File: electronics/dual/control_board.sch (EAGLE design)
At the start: 136 parts, among them J17 JST_PH_B3B-PH-K-S(LF)(SN), J18 JST_PH_B3B-PH-K-S(LF)(SN), J19 JST_PH_B3B-PH-K-S(LF)(SN), J20 JST_PH_B3B-PH-K-S(LF)(SN), J21 JST_PH_B3B-PH-K-S(LF)(SN), J22 JST_PH_B3B-PH-K-S(LF)(SN), J23 JST_PH_B3B-PH-K-S(LF)(SN), J24 JST_PH_B3B-PH-K-S(LF)(SN), J25 JST_PH_B3B-PH-K-S(LF)(SN), J26 JST_PH_B3B-PH-K-S(LF)(SN), J27 JST_PH_B3B-PH-K-S(LF)(SN), J28 JST_PH_B3B-PH-K-S(LF)(SN), J29 JST_PH_B3B-PH-K-S(LF)(SN), J30 JST_PH_B3B-PH-K-S(LF)(SN), J31 JST_PH_B3B-PH-K-S(LF)(SN), J32 JST_PH_B3B-PH-K-S(LF)(SN), J49 B4B-PH-K-S(LF)(SN), J50 B4B-PH-K-S(LF)(SN), J51 B4B-PH-K-S(LF)(SN), J52 B4B-PH-K-S(LF)(SN), J53 B4B-PH-K-S(LF)(SN), J54 B4B-PH-K-S(LF)(SN), J55 B4B-PH-K-S(LF)(SN), J56 B4B-PH-K-S(LF)(SN), J57 B4B-PH-K-S(LF)(SN), J58 B4B-PH-K-S(LF)(SN), J59 B4B-PH-K-S(LF)(SN), J60 B4B-PH-K-S(LF)(SN), J61 B4B-PH-K-S(LF)(SN), J62 B4B-PH-K-S(LF)(SN), J63 B4B-PH-K-S(LF)(SN), J64 B4B-PH-K-S(LF)(SN), Q1 BCF29SMD, U18 AD7730BRUZ, U19 AD5360BSTZ, U2 AMP-5103309-7-34PIN_5103309-7, U20 ADR425ARZ, U21 AD7730BRUZ, U23 AD7730BRUZ, U24 AD7730BRUZ, U25 AD7730BRUZ, U26 AD7730BRUZ, U27 AD7730BRUZ, U28 AD7730BRUZ, U4 ADR421ARZ, U5 AD7616BSTZ, X1 22-23-2031, Y1 KC2520B-C1, Y3 KC2520B-C1

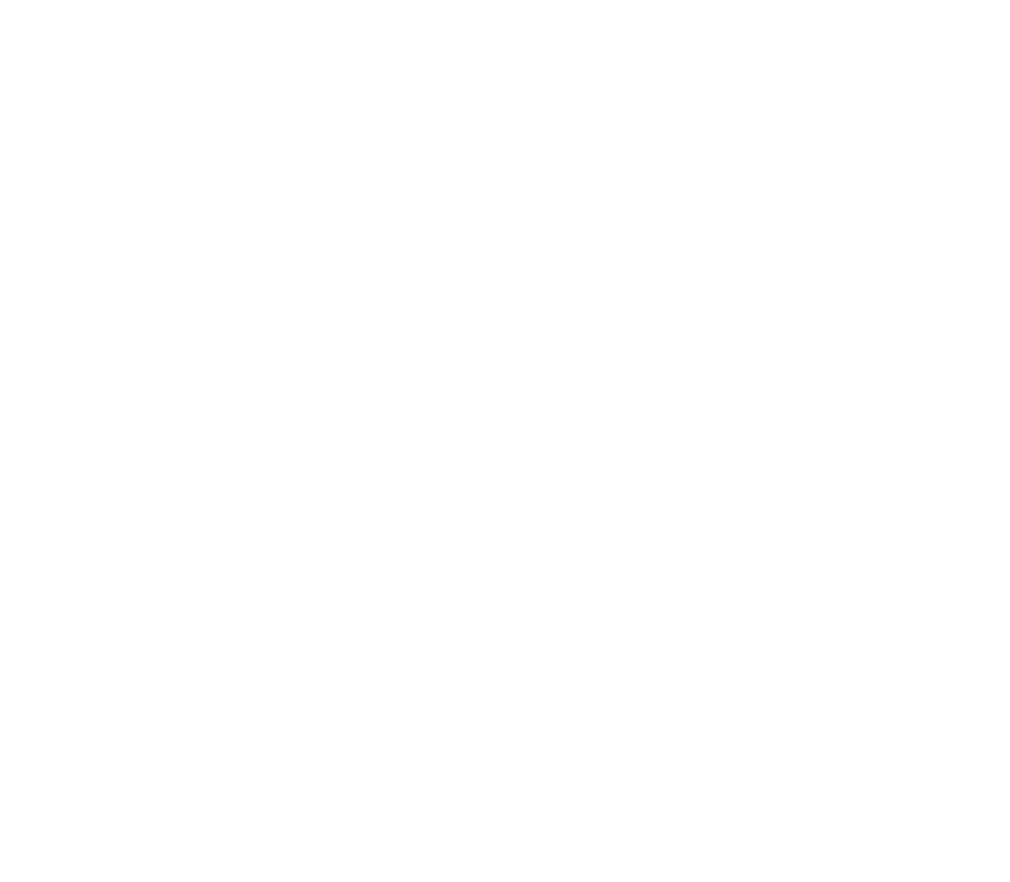
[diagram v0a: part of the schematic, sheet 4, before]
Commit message: added raspi firmware
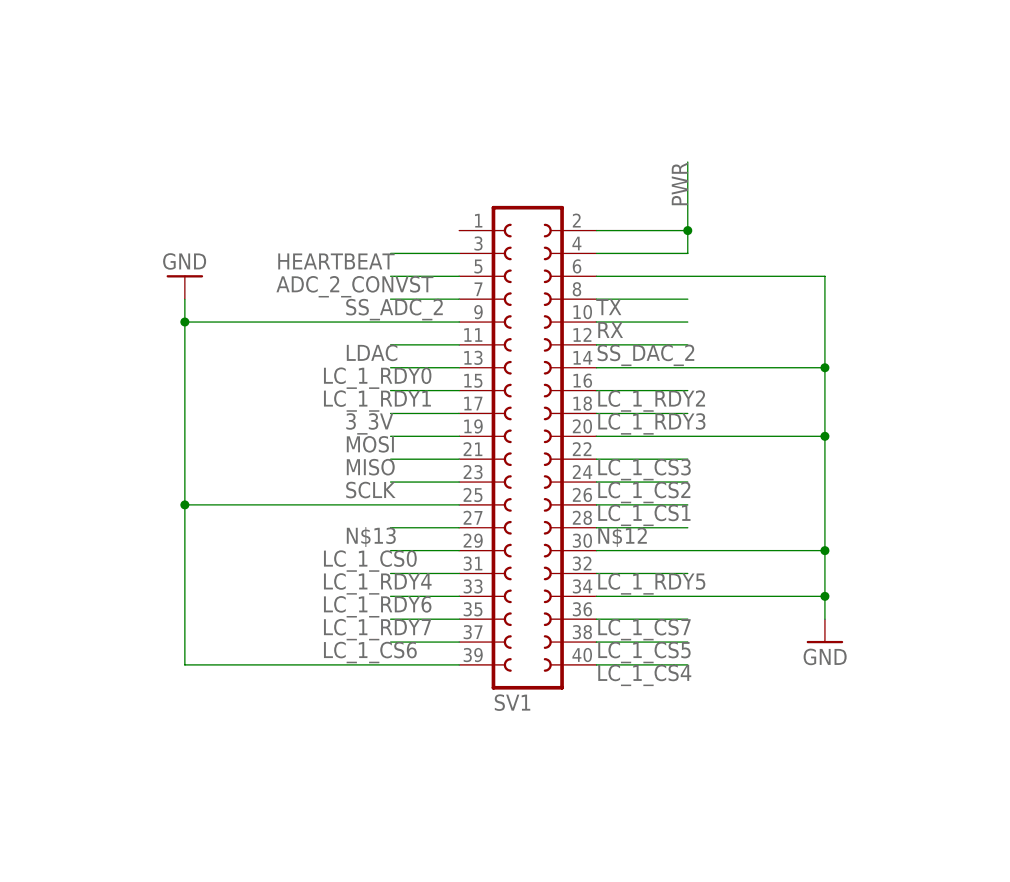
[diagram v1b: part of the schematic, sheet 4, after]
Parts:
- added SV1: (no value), con-lsta:FE20-2
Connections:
- new net 3_3V: SV1.17
- new net N$12: SV1.28
- new net N$13: SV1.27
- net ADC_2_CONVST: now also SV1.5
- net GND: now also SV1.14, SV1.20, SV1.25, SV1.30, SV1.34, SV1.39, SV1.6, SV1.9
- net HEARTBEAT: now also SV1.3
- net LC_1_CS0: now also SV1.29
- net LC_1_CS1: now also SV1.26
- net LC_1_CS2: now also SV1.24
- net LC_1_CS3: now also SV1.22
- net LC_1_CS4: now also SV1.40
- net LC_1_CS5: now also SV1.38
- net LC_1_CS6: now also SV1.37
- net LC_1_CS7: now also SV1.36
- net LC_1_RDY0: now also SV1.13
- net LC_1_RDY1: now also SV1.15
- net LC_1_RDY2: now also SV1.16
- net LC_1_RDY3: now also SV1.18
- net LC_1_RDY4: now also SV1.31
- net LC_1_RDY5: now also SV1.32
- net LC_1_RDY6: now also SV1.33
- net LC_1_RDY7: now also SV1.35
- net LDAC: now also SV1.11
- net MISO: now also SV1.21
- net MOSI: now also SV1.19
- net PWR: now also SV1.2, SV1.4
- net RX: now also SV1.10
- net SCLK: now also SV1.23
- net SS_ADC_2: now also SV1.7
- net SS_DAC_2: now also SV1.12
- net TX: now also SV1.8
